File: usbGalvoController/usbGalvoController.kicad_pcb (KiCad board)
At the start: 2 copper layers, 40.6 x 43.2 mm, 26 parts, among them P1 USB_OTG, P2 CONN_01X06, P3 GND, P4 PWR, P5 DAC, P6 GPIO, P7 UART, U1 STM32L151x6, U2 LD1117S33CTR, Y1 8MHz

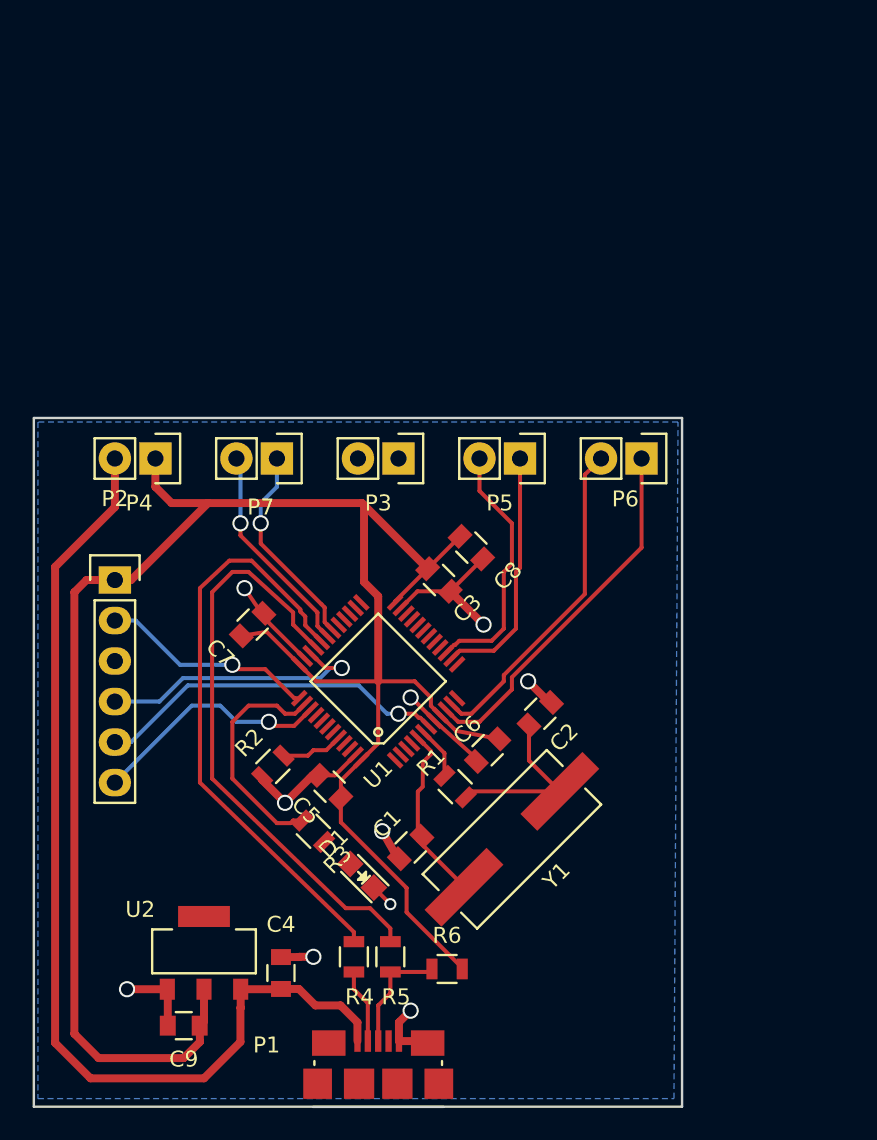
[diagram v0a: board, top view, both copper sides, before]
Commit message: Finished layout for usbGalvoController v0.2
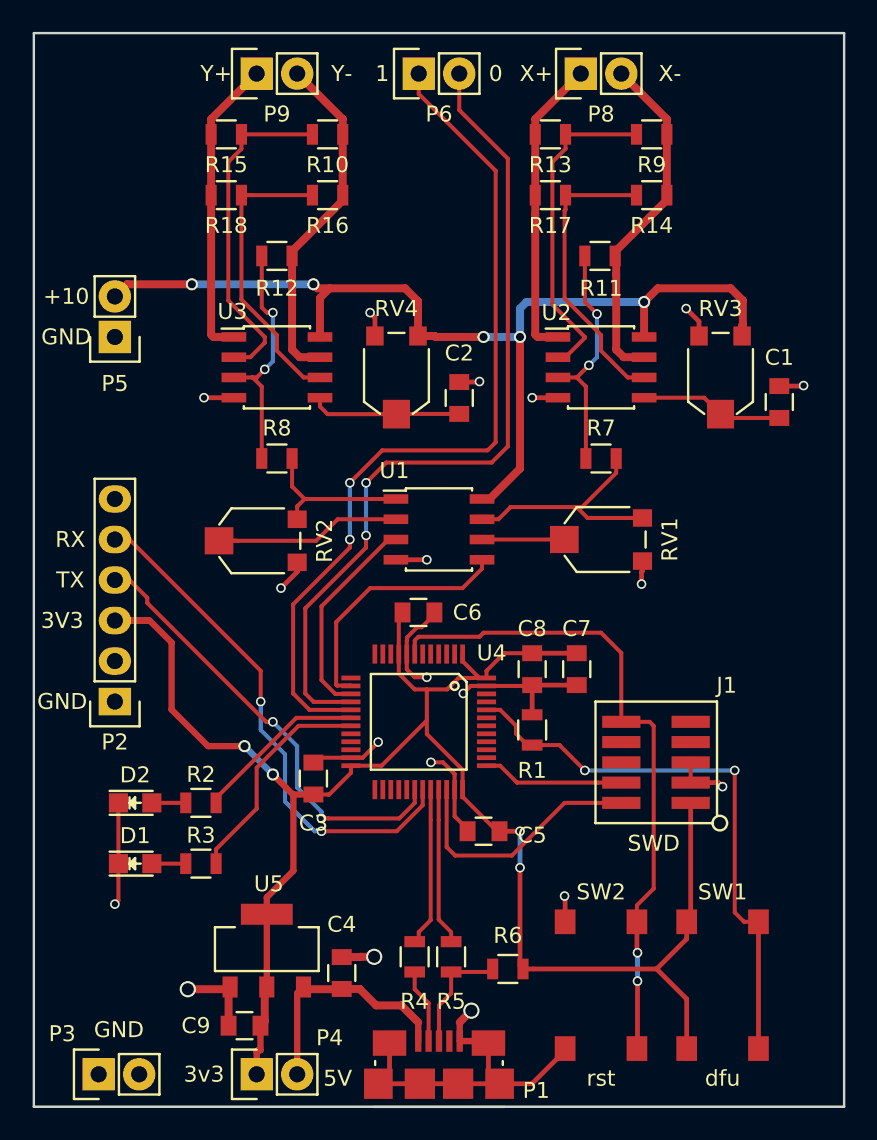
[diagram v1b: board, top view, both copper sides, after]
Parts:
- removed P7: UART, Pin_Headers:Pin_Header_Straight_1x02
- removed Y1: 8MHz, alvarop:ATS-SM-CRYSTAL
- added D2: LED, LEDs:LED_0805, F.Cu at (133.3, 108.0)
- added J1: ARM-SWD, footprints:ARM_SWD_SMD, F.Cu at (166.0, 105.4)
- added P8: X_OUT, Pin_Headers:Pin_Header_Straight_1x02, F.Cu at (161.3, 62.2)
- added P9: Y_OUT, Pin_Headers:Pin_Header_Straight_1x02, F.Cu at (141.0, 62.2)
- added R10: 2.21k, Resistors_SMD:R_0805, F.Cu at (145.4, 66.0)
- added R11: 10k, Resistors_SMD:R_0805, F.Cu at (162.5, 73.7)
- added R12: 10k, Resistors_SMD:R_0805, F.Cu at (142.2, 73.7)
- added R13: 2.21k, Resistors_SMD:R_0805, F.Cu at (159.4, 66.0)
- added R14: 2.21k, Resistors_SMD:R_0805, F.Cu at (165.7, 69.8)
- added R15: 2.21k, Resistors_SMD:R_0805, F.Cu at (139.1, 66.0)
- added R16: 2.21k, Resistors_SMD:R_0805, F.Cu at (145.4, 69.8)
- added R17: 2.21k, Resistors_SMD:R_0805, F.Cu at (159.4, 69.8)
- added R18: 2.21k, Resistors_SMD:R_0805, F.Cu at (139.1, 69.8)
- added R7: 10k, Resistors_SMD:R_0805, F.Cu at (162.6, 86.4)
- added R8: 10k, Resistors_SMD:R_0805, F.Cu at (142.2, 86.4)
- added R9: 2.21k, Resistors_SMD:R_0805, F.Cu at (165.7, 66.0)
- added RV1: POT, alvarop:POT-4mm, F.Cu at (162.6, 91.4)
- added RV2: POT, alvarop:POT-4mm, F.Cu at (140.9, 91.5)
- added RV3: POT, alvarop:POT-4mm, F.Cu at (170.1, 81.3)
- added RV4: POT, alvarop:POT-4mm, F.Cu at (149.7, 81.3)
- added SW1: BOOT, footprints:PTS645SM43SMTR92, F.Cu at (170.2, 119.4)
- added SW2: RST, footprints:PTS645SM43SMTR92, F.Cu at (162.6, 119.4)
- added U3: LM358, Housings_SOIC:SOIC-8_3.9x4.9mm_Pitch1.27mm, F.Cu at (142.2, 80.6)
- added U4: stm32f072x, footprints:LQFP48, F.Cu at (151.1, 102.9)
- added U5: LD1117S33CTR, alvarop:SOT-223, F.Cu at (141.6, 119.5)
- C1, C2: value 20pF -> 100nF
- D1: footprint LEDs:LED-0805 -> LEDs:LED_0805
- P5: value DAC -> A_PWR
- R1: value 390 -> 10k
- R2: value 10k -> 680
- U1: value STM32L151x6 -> LM358; footprint alvarop:LQFP48 -> Housings_SOIC:SOIC-8_3.9x4.9mm_Pitch1.27mm
- U2: value LD1117S33CTR -> LM358; footprint alvarop:SOT-223 -> Housings_SOIC:SOIC-8_3.9x4.9mm_Pitch1.27mm
- moved U2 46.3 mm to (162.6, 80.6)
- moved P3 42.9 mm to (131.1, 125.0), turned to 90 degrees
- moved P4 39.1 mm to (141.0, 125.0), turned to 90 degrees
- moved C1 36.2 mm to (173.7, 82.8), turned to 90 degrees
- moved P6 27.9 mm to (151.1, 62.2), turned to 90 degrees
- moved P5 26.5 mm to (132.1, 78.7), turned to 180 degrees
- moved C7 20.5 mm to (161.0, 99.6), turned to 270 degrees
- moved C2 20.4 mm to (153.7, 82.6), turned to 90 degrees
- moved C3 14.7 mm to (144.5, 106.4), turned to 90 degrees
- moved D1 14.2 mm to (133.3, 111.8), turned to 0 degrees
- moved U1 10.3 mm to (152.4, 90.8), turned to 0 degrees
- moved C5 10.0 mm to (155.2, 109.7), turned to 180 degrees
- moved C6 9.66 mm to (151.1, 96.0), turned to 0 degrees
- moved C8 8.52 mm to (158.2, 99.6), turned to 270 degrees
- moved P2 7.62 mm to (132.1, 101.6), turned to 180 degrees
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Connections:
- C1 pad 1: GND -> Net-(C1-Pad1)
- C1 pad 2: Net-(C1-Pad2) -> GND
- C2 pad 1: GND -> Net-(C2-Pad1)
- C2 pad 2: Net-(C2-Pad2) -> GND
- P2 pad 1: +3V3 -> GND
- P2 pad 2: /SWCLK -> Net-(P2-Pad2)
- P2 pad 3: GND -> +3V3
- P2 pad 4: /SWDIO -> /UART1_TX
- P2 pad 5: /nRST -> /UART1_RX
- P2 pad 6: /SWO -> Net-(P2-Pad6)
- P5 pad 1: /DAC1 -> GND
- P5 pad 2: /DAC2 -> VDD
- P6 pad 1: /GPIO0 -> /GPIO1
- P6 pad 2: /GPIO1 -> /GPIO0
- R1 pad 1: Net-(C2-Pad2) -> /boot0
- R1 pad 2: Net-(R1-Pad2) -> GND
- R2 pad 1: GND -> /LED0
- R2 pad 2: Net-(R2-Pad2) -> Net-(D2-Pad2)
- R3 pad 1: Net-(R3-Pad1) -> /LED1
- U1 pad 3: Net-(U1-Pad3) -> /DAC2
- U1 pad 4: Net-(U1-Pad4) -> GND
- U1 pad 5: Net-(C1-Pad2) -> /DAC1
- U1 pad 6: Net-(R1-Pad2) -> Net-(RV1-Pad2)
- U1 pad 7: /nRST -> Net-(R7-Pad2)
- U1 pad 8: GND -> VDD
- U2 pad 1: GND -> /XOUT_P
- U2 pad 2: +3V3 -> Net-(R13-Pad2)
- U2 pad 3: +5V -> Net-(R11-Pad2)
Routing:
- net VDD: track 0.00 -> 64.1 mm, vias 0 -> 5
- net +5V: track 64.4 -> 15.0 mm
- net GND: track 45.4 -> 81.6 mm, vias 10 -> 19
- net /boot0: track 0.00 -> 36.0 mm, vias 0 -> 2
- net /GPIO1: track 20.9 -> 54.0 mm, vias 0 -> 2
- net /UART1_RX: track 0.00 -> 32.6 mm, vias 0 -> 2
- net /GPIO0: track 23.1 -> 52.3 mm, vias 0 -> 2
- net /UART1_TX: track 0.00 -> 28.4 mm, vias 0 -> 2
- net /DM: track 37.1 -> 9.95 mm
- net /DP: track 36.9 -> 9.86 mm
- net /XOUT_M: track 0.00 -> 22.0 mm
- net /YOUT_M: track 0.00 -> 21.7 mm
- net Net-(R10-Pad2): track 0.00 -> 21.1 mm
- net Net-(R13-Pad2): track 0.00 -> 20.6 mm
- net /nRST: track 22.2 -> 42.4 mm, vias 1 -> 2
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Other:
- board size 40.6 x 43.2 mm -> 50.8 x 67.3 mm
- board text added: "+10"
- board text added: "0"
- board text added: "1"
- board text added: "3V3"
- board text added: "3v3"
- board text added: "5V"
- board text added: "GND"
- board text added: "RX"
- board text added: "SWD"
- board text added: "TX"
- board text added: "X+"
- board text added: "X-"
- board text added: "Y+"
- board text added: "Y-"
- board text added: "dfu"
- board text added: "rst"
- board text added: "usbGalvoController v0.2 by @alvaroprieto"
- board text removed: "dac"
- board text removed: "gnd"
- board text removed: "gpio"
- board text removed: "pwr"
- board text removed: "uart"
- board text removed: "usbGalvoController v0.1 by @alvaroprieto"
